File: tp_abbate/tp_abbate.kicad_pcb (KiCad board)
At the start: 2 copper layers, 43 x 61.5 mm, 45 parts, among them J101 USB_B_Micro, J102 S2B-PH-K-S, J201 U.FL-R-SMT-1(10), J202 Conn_01x06, J203 Conn_01x12, J204 Conn_01x12, Q101 AO3401A, Q201 AO3401A, Q202 2N7002DW, SW201 SW_Push, SW202 SW_Push, U101 LTC4054ES5-4.2, U102 CP2102-GM-QFN28, U103 MIC5219-3.3YMM, U201 ESP32-WROOM-32, U202 Ai-Thinker-Ra-01

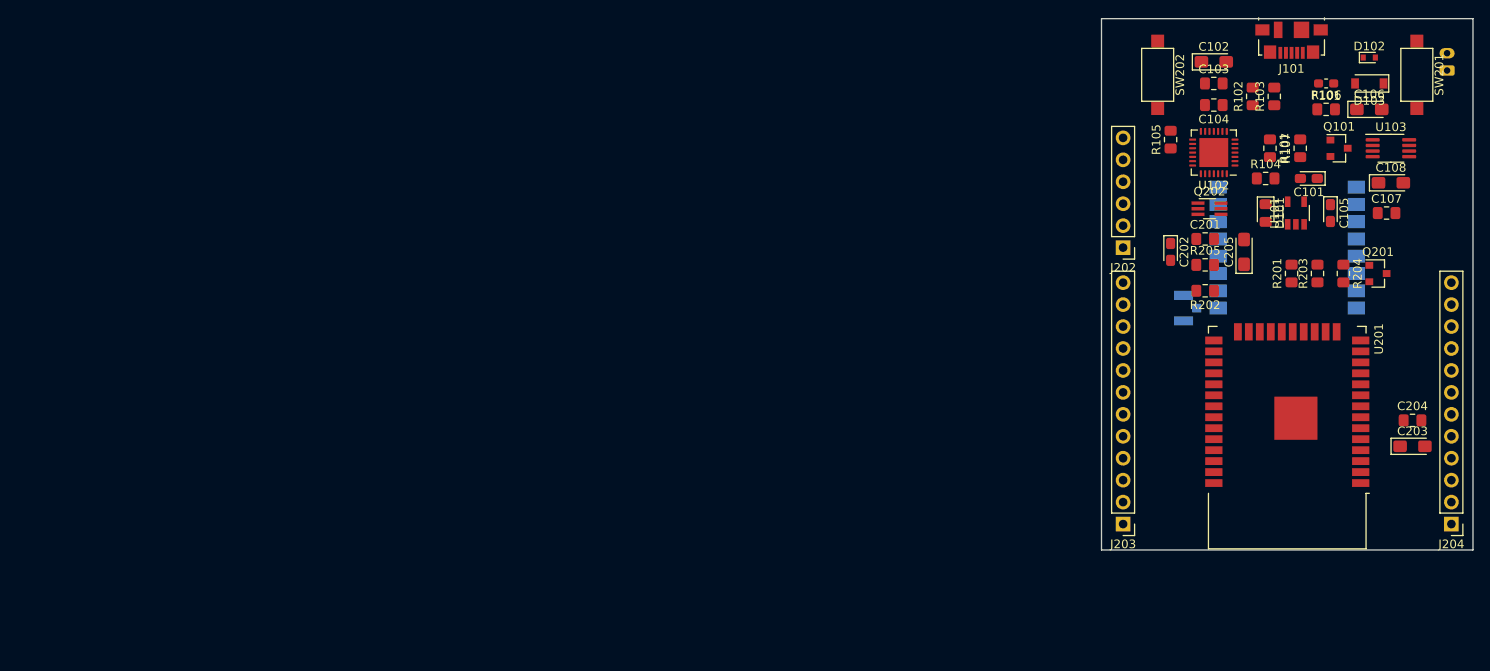
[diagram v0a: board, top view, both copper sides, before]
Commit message: WIP revisión PCB
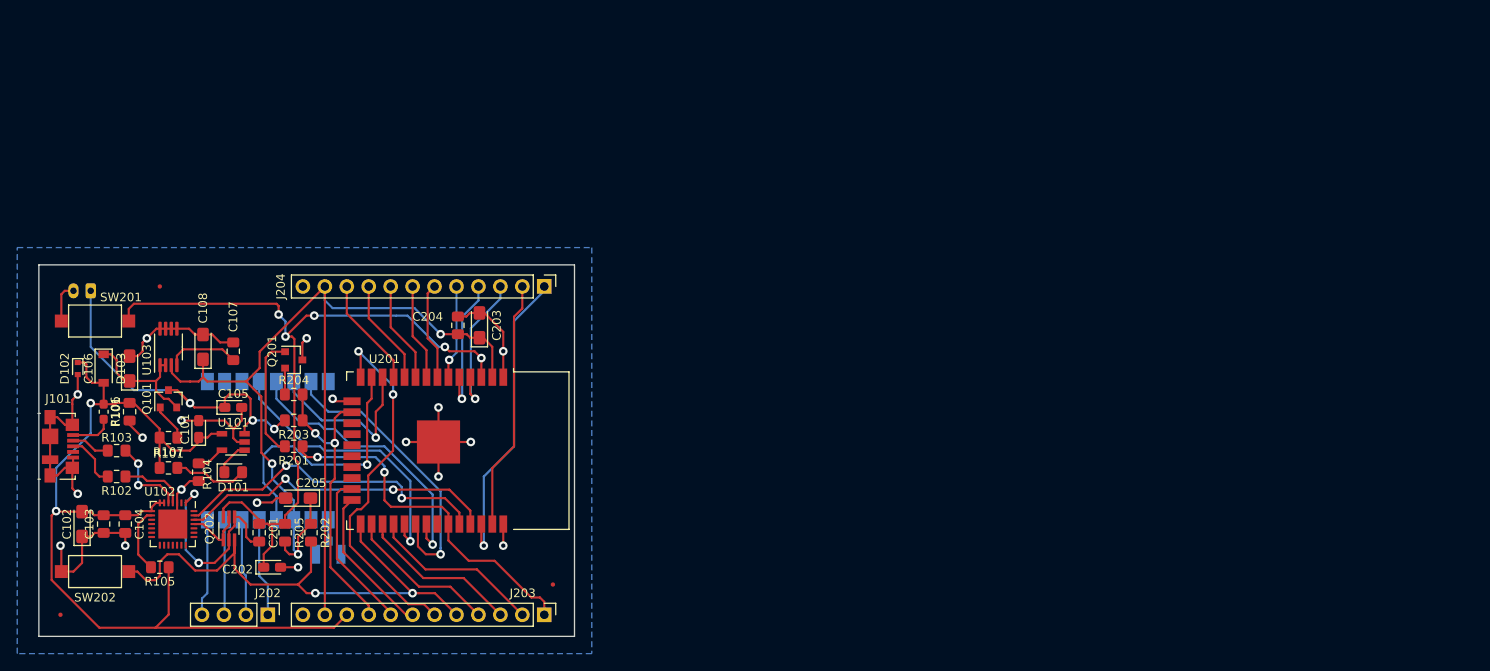
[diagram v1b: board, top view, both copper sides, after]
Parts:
- added FID1: Fiducial, Fiducial:Fiducial_0.5mm_Mask1.5mm, F.Cu at (89.0, 118.5)
- added FID2: Fiducial, Fiducial:Fiducial_0.5mm_Mask1.5mm, F.Cu at (100.5, 80.5)
- added FID3: Fiducial, Fiducial:Fiducial_0.5mm_Mask1.5mm, F.Cu at (146.0, 115.0)
- J202: value Conn_01x06 -> Conn_01x04; footprint Connector_PinHeader_2.54mm:PinHeader_1x06_P2.54mm_Vertical -> Connector_PinHeader_2.54mm:PinHeader_1x04_P2.54mm_Vertical
- moved J102 159.1 mm to (92.5, 81.0), turned to 180 degrees
- moved SW201 155.6 mm to (93.0, 84.5), turned to 0 degrees
- moved D102 153.8 mm to (91.0, 90.0), turned to 270 degrees
- moved D103 150.2 mm to (94.0, 90.0), turned to 270 degrees
- moved J101 150.1 mm to (89.0, 99.0), turned to 270 degrees
- moved C106 146.6 mm to (97.0, 90.0), turned to 90 degrees
- moved F101 146.5 mm to (94.0, 95.0), turned to 270 degrees
- moved U103 143.4 mm to (101.5, 87.5), turned to 90 degrees
- moved R106 142.9 mm to (97.0, 95.0), turned to 90 degrees
- moved C102 141.5 mm to (91.5, 108.0), turned to 90 degrees
- moved R103 140.1 mm to (95.5, 99.5), turned to 180 degrees
- moved C108 138.8 mm to (105.5, 87.5), turned to 90 degrees
- moved R102 138.7 mm to (95.5, 102.5), turned to 180 degrees
- moved Q101 138.6 mm to (101.5, 93.5), turned to 90 degrees
- moved C103 138.3 mm to (94.0, 108.0), turned to 90 degrees
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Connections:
- J203 pad 6: /ESP32/GPIO2 -> /ESP32/GPIO12
- J203 pad 7: /ESP32/GPIO15 -> /ESP32/GPIO2
- J203 pad 8: /ESP32/GPIO13 -> /ESP32/GPIO15
- J203 pad 9: /ESP32/GPIO12 -> /ESP32/GPIO13
- U202 pad 10: Net-(J202-Pad5) -> Net-(U202-Pad10)
- U202 pad 11: Net-(J202-Pad6) -> Net-(U202-Pad11)
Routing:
- net +3V3: track 0.00 -> 124.0 mm, vias 0 -> 3
- net GND: track 0.00 -> 119.3 mm, vias 0 -> 18
- net +5V: track 0.00 -> 110.7 mm, vias 0 -> 2
- net /ESP32/CHIP_PU: track 0.00 -> 90.8 mm, vias 0 -> 5
- net /ESP32/GPIO0: track 0.00 -> 65.3 mm, vias 0 -> 2
- net +BATT: track 0.00 -> 43.7 mm, vias 0 -> 3
- net /ESP32/GPIO12: track 0.00 -> 42.7 mm, vias 0 -> 2
- net /ESP32/GPIO21: track 0.00 -> 42.0 mm, vias 0 -> 2
- net /ESP_RXD: track 0.00 -> 37.4 mm, vias 0 -> 2
- net /ESP_TXD: track 0.00 -> 37.0 mm, vias 0 -> 2
- net /ESP32/GPIO22: track 0.00 -> 35.5 mm, vias 0 -> 1
- net /ESP32/GPIO13: track 0.00 -> 34.9 mm, vias 0 -> 2
- net /ESP32/LORA_SS: track 0.00 -> 34.1 mm, vias 0 -> 1
- net /ESP32/LORA_MISO: track 0.00 -> 33.1 mm, vias 0 -> 1
- net /ESP32/LORA_SCK: track 0.00 -> 32.7 mm, vias 0 -> 1
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- added copper zone on B.Cu, net GND
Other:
- board size 43 x 61.5 mm -> 62 x 43 mm
- net class Default: via_dia 1.27 -> 1; via_drill 0.7 -> 0.5
- net class USB_Conn: via_dia 1.27 -> 1; via_drill 0.7 -> 0.5
- rule pad_to_mask_clearance: 0.05 -> 0.1
- board text added: "Grillas: - Principal 0,5mm - Alternativa 0,25mm Separación al borde: 0,5mm Estándar de fabricación: http://www.mayerpcb.com/uploads/estandares.pdf Net class "Default" : Mayer 10 mils - Ancho mínimo de traza 0,25mm - Separacion mínima entre trazas 0,25mm - Diametro mínimo de via 1mm - Perforación mínima de via 0,5m Net class "USB_Conn" : Mayer 8 mils - Ancho mínimo de traza 0,2mm - Separacion míni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"
- board text added: "Reglas de diseño y fabricación"
